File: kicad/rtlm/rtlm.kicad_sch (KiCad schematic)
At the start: 66 parts, among them IC1 ESP32-S3FN8, IC2 TPS25940ARVCR, IC3 PE4259, J1 USB_C_Receptacle_USB2.0_16P, J2 Conn_01x02, J3 UART_DEBUG_3V3, Q1 DMP2035U-7, SW1 SW_Push, SW2 SW_Push, U1 TPS62130A, U2 TPS2116DRL, U3 TPD2EUSB30, U4 SX1262IMLTRT, Y1 40MHz, Y2 TG2520SMN 32.0000M-MCGNNM3

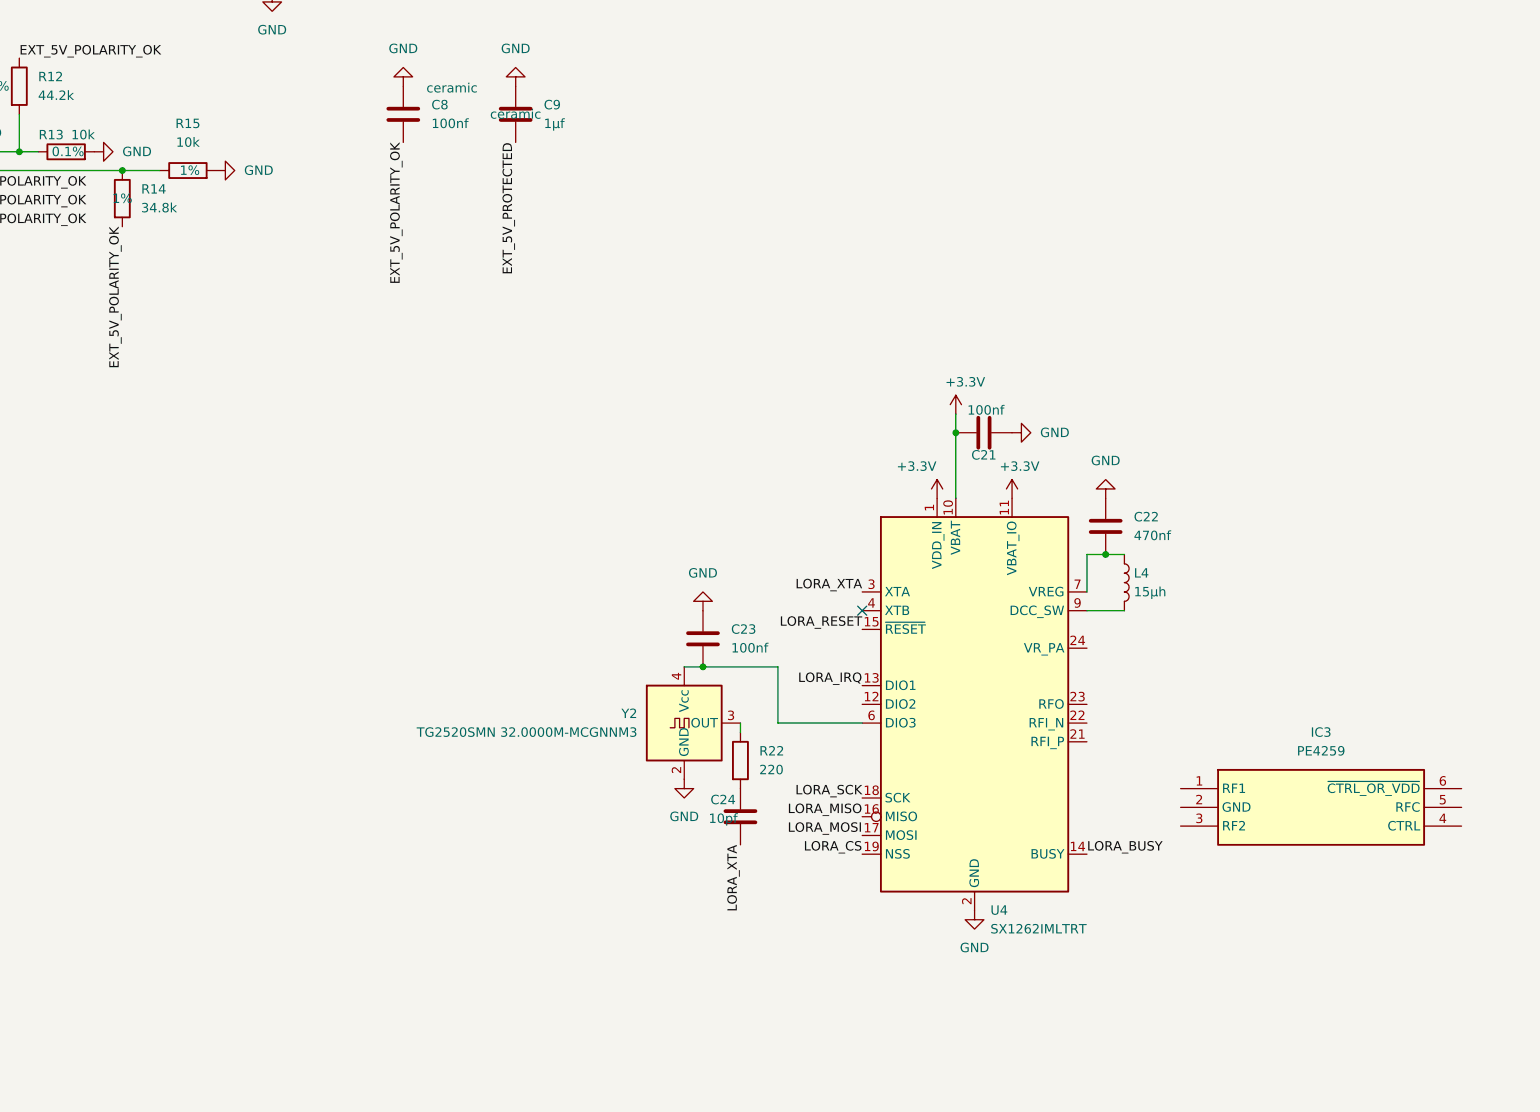
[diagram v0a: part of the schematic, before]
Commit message: feat: basic LoRa module complete
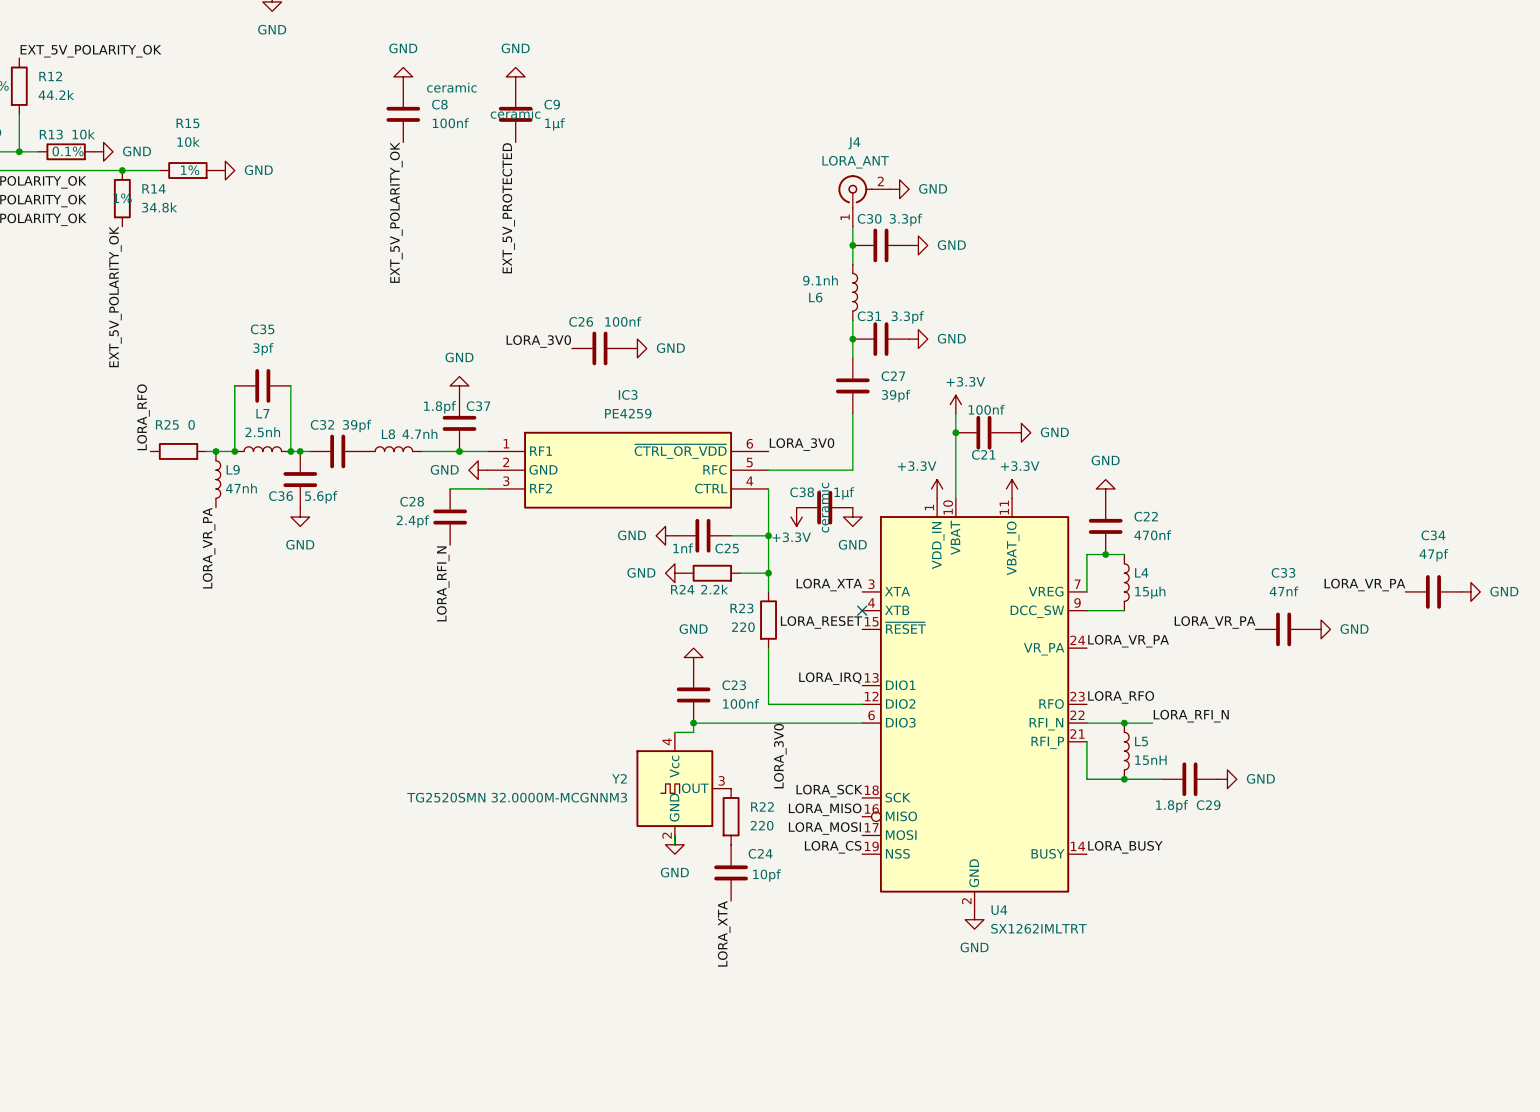
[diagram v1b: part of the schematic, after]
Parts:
- added C25: 1nf, symbol Device:C
- added C26: 100nf, symbol Device:C
- added C27, C32: 39pf, symbol Device:C
- added C28: 2.4pf, symbol Device:C
- added C29, C37: 1.8pf, symbol Device:C
- added C30, C31: 3.3pf, symbol Device:C
- added C33: 47nf, symbol Device:C
- added C34: 47pf, symbol Device:C
- added C35: 3pf, symbol Device:C
- added C36: 5.6pf, symbol Device:C
- added C38: 1µf, symbol Device:C
- added J4: LORA_ANT, Connector_Coaxial:U.FL_Hirose_U.FL-R-SMT-1_Vertical, symbol Connector:Conn_Coaxial
- added L5: 15nH, symbol Device:L
- added L6: 9.1nh, symbol Device:L
- added L7: 2.5nh, symbol Device:L
- added L8: 4.7nh, symbol Device:L
- added L9: 47nh, symbol Device:L
- added R23: 220, symbol Device:R
- added R24: 2.2k, symbol Device:R
- added R25: 0, symbol Device:R
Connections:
- net +3.3V: now also C38.1
- net GND: now also IC3.2 (GND), C25.1, C26.1, C29.1, C30.2, C31.2, C33.2, C34.2, C36.2, C37.2, C38.2, J4.2 (Ext), R24.1
- net at U4.12 (DIO2): now also R23.2
- net at U4.21 (RFI_P): now also C29.2, L5.2
- net LORA_RFI_N: now reaches U4.22 (RFI_N)
- net LORA_RFI_N: now also C28.2, L5.1
- net LORA_RFO: now reaches U4.23 (RFO)
- net LORA_RFO: now also R25.1
- net LORA_VR_PA: now reaches U4.24 (VR_PA)
- net LORA_VR_PA: now also C33.1, C34.1, L9.2
- net LORA_3V0: now reaches C23.2, U4.6 (DIO3), Y2.4 (Vcc)
- net LORA_3V0: now also IC3.6 (~{CTRL_OR_VDD}), C26.2
- net at IC3.1 (RF1): now also C37.1, L8.2
- net at IC3.3 (RF2): now also C28.1
- net at IC3.4 (CTRL): now also C25.2, R23.1, R24.2
- net at IC3.5 (RFC): now also C27.2
- new net: C27.1, C31.1, L6.2
- new net: C32.2, L8.1
- new net: C35.1, L7.1, L9.1, R25.2
- new net: C30.1, J4.1 (In), L6.1
- new net: C32.1, C35.2, C36.1, L7.2
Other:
- moved on the sheet: C23, C24, IC3, R22, Y2
